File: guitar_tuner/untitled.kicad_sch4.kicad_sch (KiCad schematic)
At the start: 7 parts, among them U3 EA OLEDM128-6LWA

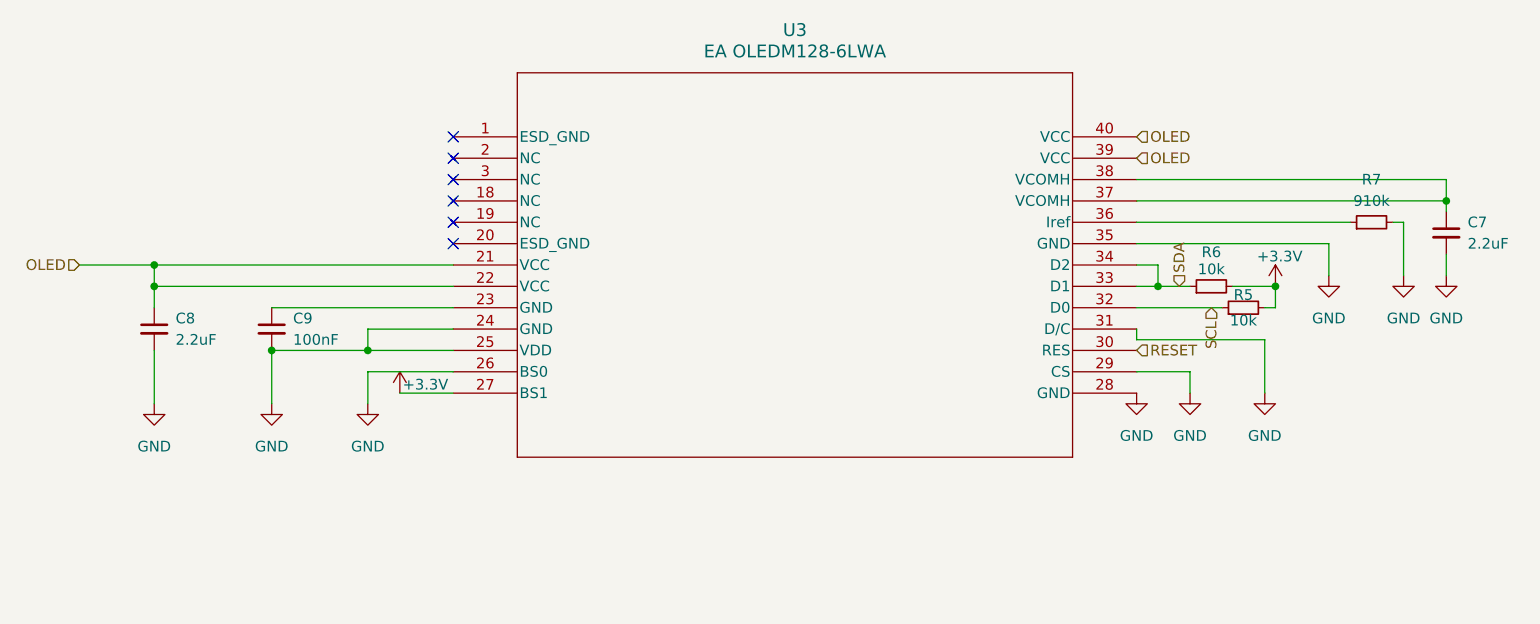
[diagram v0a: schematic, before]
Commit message: Screen
New Screen
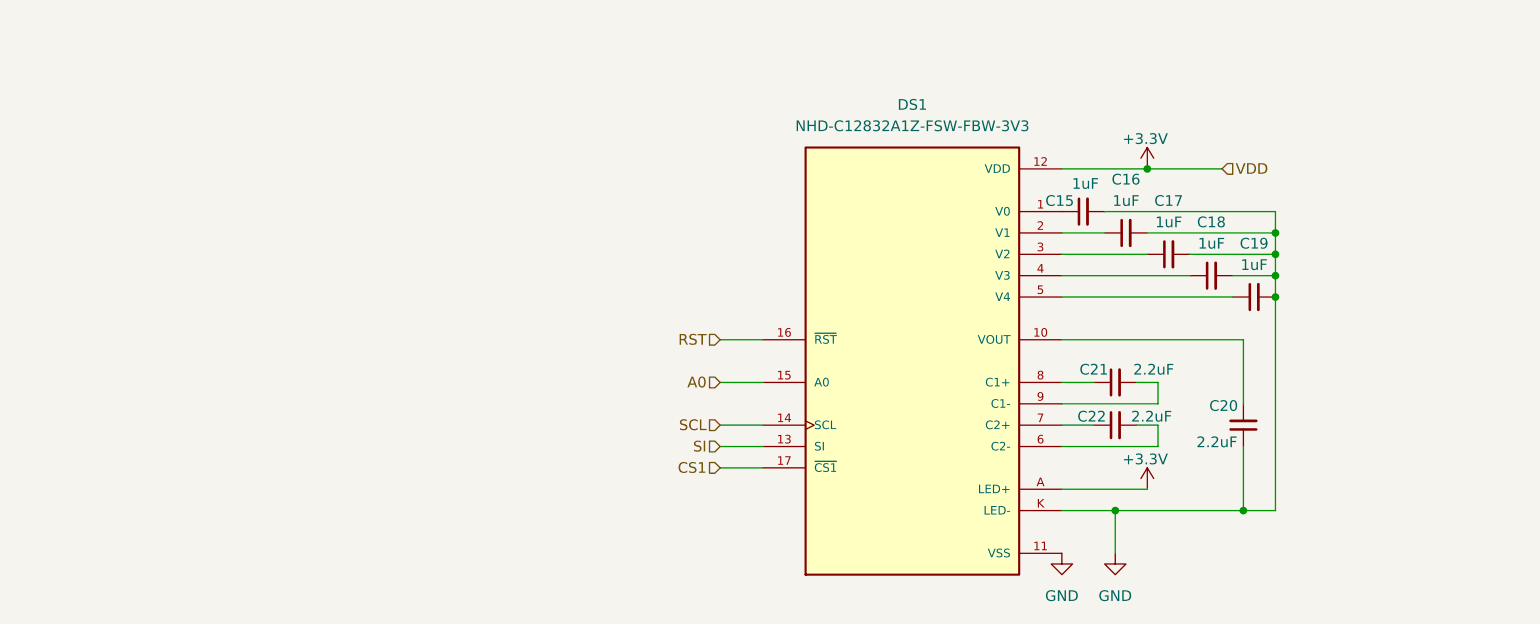
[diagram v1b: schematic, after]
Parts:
- removed C7, C8: 2.2uF, symbol Device:C_Small
- removed C9: 100nF, symbol Device:C_Small
- removed R5, R6: 10k, symbol Device:R_Small
- removed R7: 910k, symbol Device:R_Small
- removed U3: EA OLEDM128-6LWA, DIP40_EA OLEDM128-6LWA_ELC, symbol 2025-03-15_02-14-28:EA_OLEDM128-6LWA
- added C15, C16, C17, C18, C19: 1uF, symbol Device:C_Small
- added C20, C21, C22: 2.2uF, symbol Device:C_Small
- added DS1: NHD-C12832A1Z-FSW-FBW-3V3, NHD-C12832A1Z-FSW-FBW-3V3:LCD_NHD-C12832A1Z-FSW-FBW-3V3, symbol NHD-C12832A1Z-FSW-FBW-3V3:NHD-C12832A1Z-FSW-FBW-3V3
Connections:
- net +3.3V: now also DS1.12 (VDD), DS1.A (LED+)
- net GND: now also C15.2, C16.2, C17.2, C18.2, C19.2, C20.1, DS1.11 (VSS), DS1.K (LED-)
- net SCL: now also DS1.14 (SCL)
- new net: C18.1, DS1.4 (V3)
- new net: C20.2, DS1.10 (VOUT)
- new net: C17.1, DS1.3 (V2)
- new net: C15.1, DS1.1 (V0)
- new net: C16.1, DS1.2 (V1)
- new net: C19.1, DS1.5 (V4)
- new net: C22.2, DS1.6 (C2-)
- new net: C22.1, DS1.7 (C2+)
- new net: C21.1, DS1.8 (C1+)
- new net: C21.2, DS1.9 (C1-)
- new net A0: DS1.15 (A0)
- new net CS1: DS1.17 (~{CS1})
- new net RST: DS1.16 (~{RST})
- new net SI: DS1.13 (SI)
- no-connect marks 6 -> 0
